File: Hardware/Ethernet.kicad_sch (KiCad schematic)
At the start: 39 parts, among them J1 Conn_01x07_Male, J10 SPI, J2 Conn_01x04_Male, J3 Conn_01x02_Male, J4 Conn_01x02_Male, J5 Conn_01x02_Male, J6 Conn_01x02_Male, J7 Conn_01x08_Male, J8 SPI, J9 QWIIC_Stackable, U1 W5500, Y1 25MHz_SMD_Crystal_Resonator

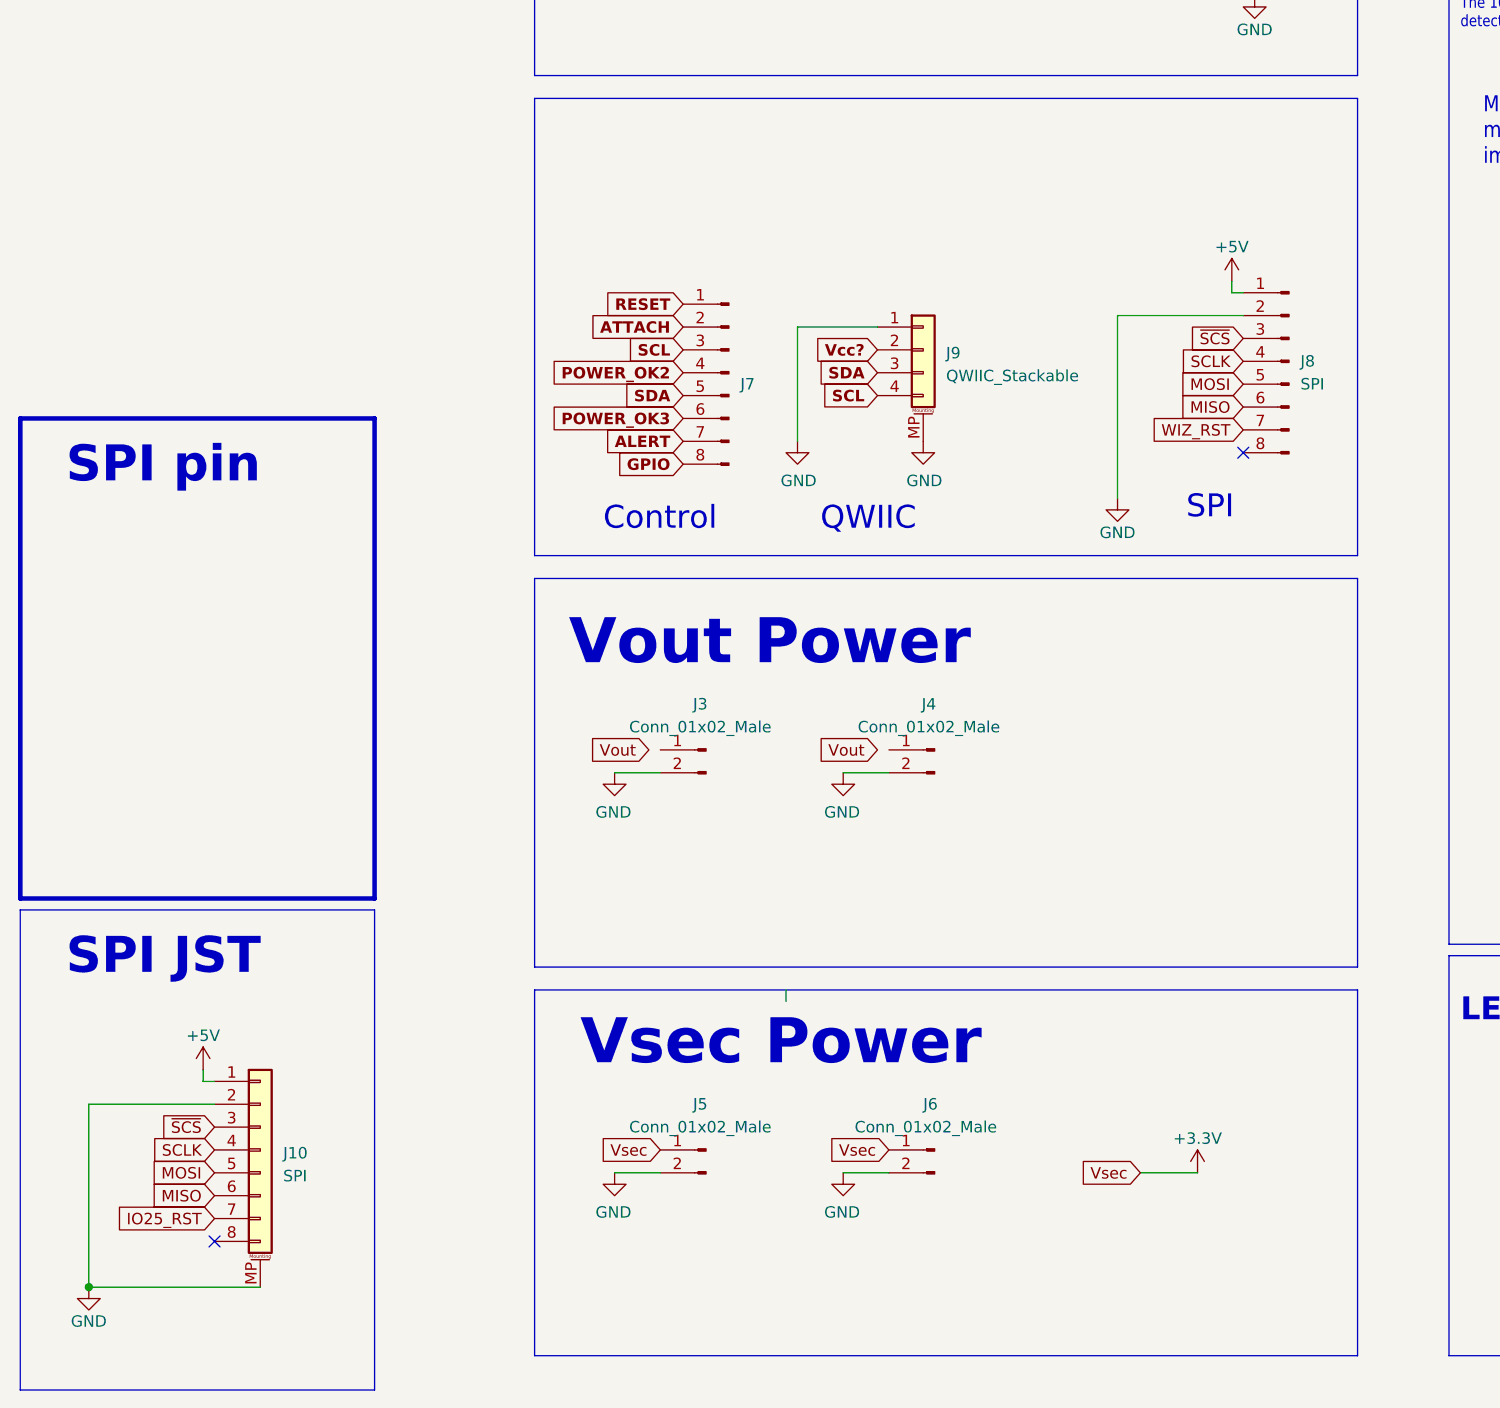
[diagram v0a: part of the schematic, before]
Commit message: Working on SPI
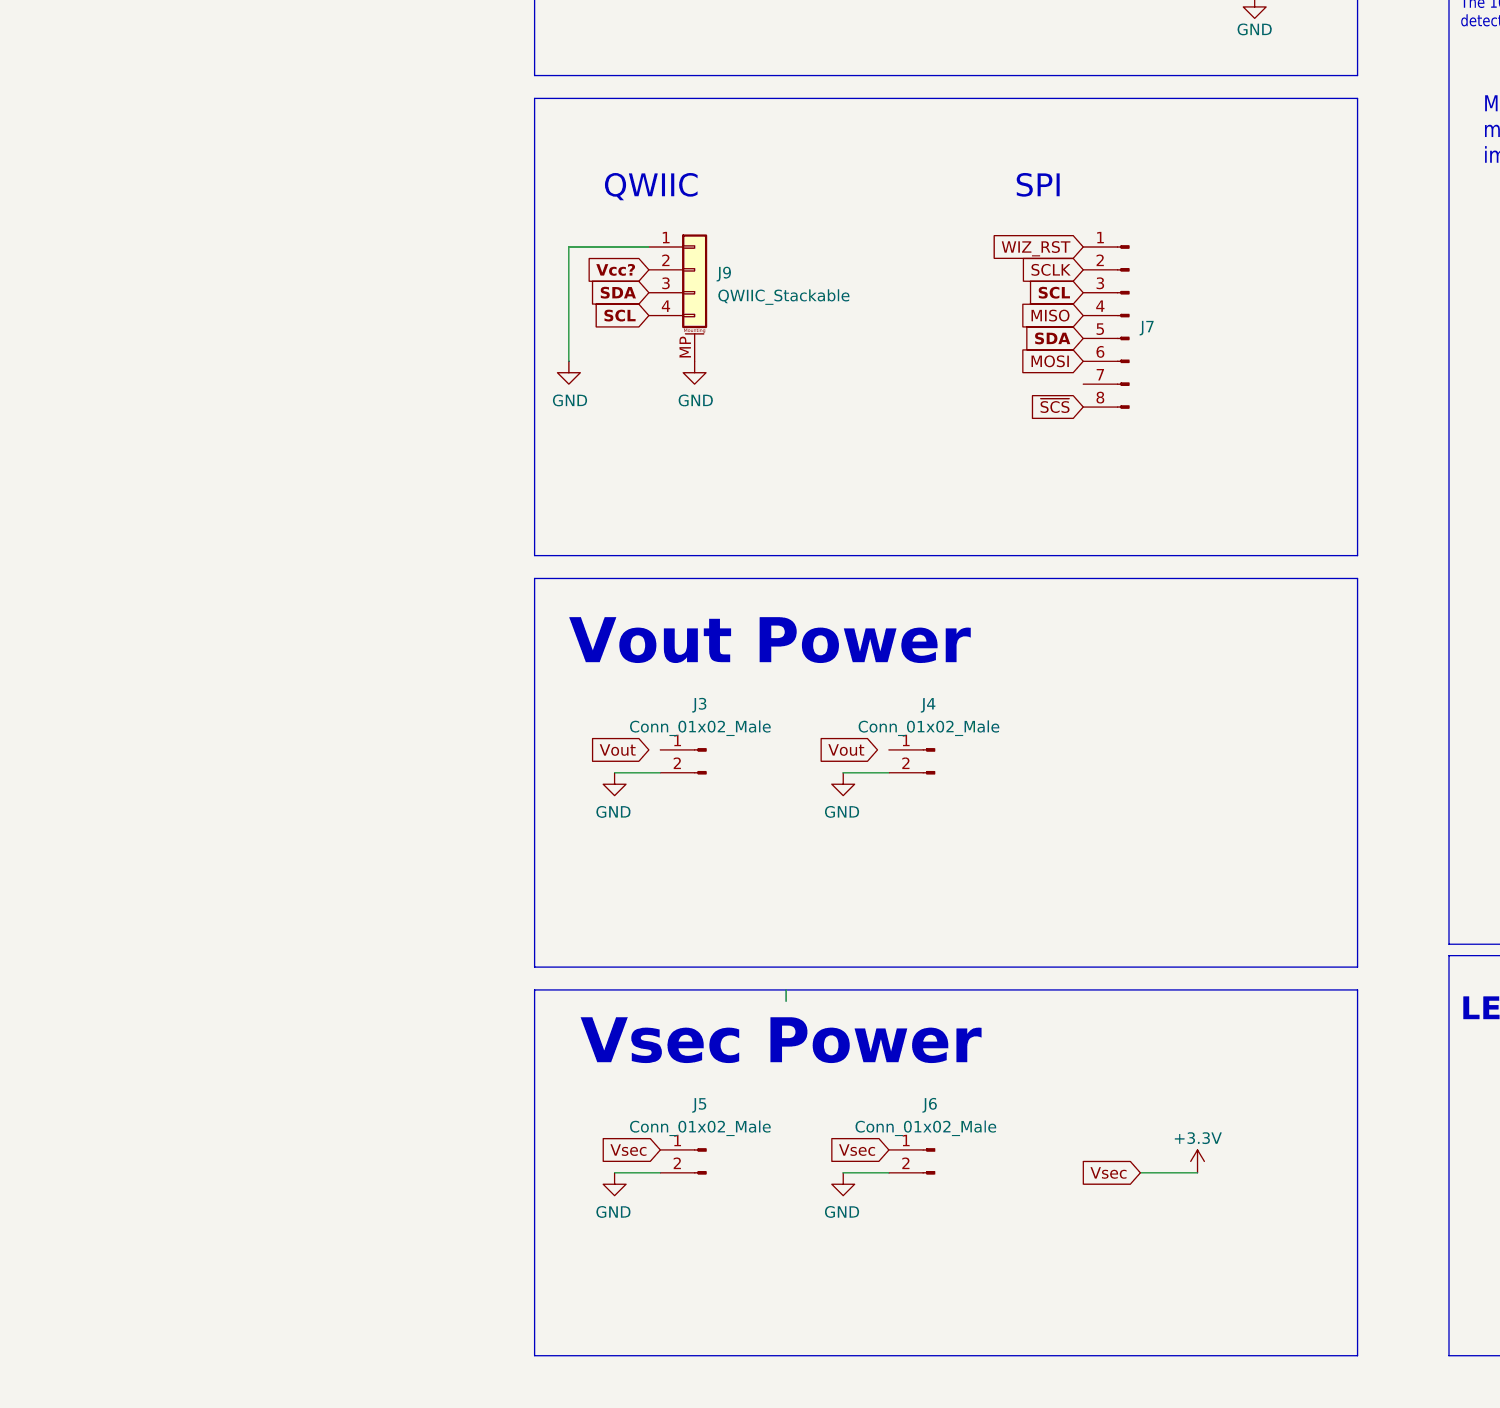
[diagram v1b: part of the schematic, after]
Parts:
- removed J10: SPI, bare-footprints:8 pin jst 1.25 vertical, symbol Connector_Generic_MountingPin:Conn_01x08_MountingPin
- removed J8: SPI, Tinker:PinHeader_1x08_P1.27mm_Vertical, symbol Connector:Conn_01x08_Male
- J7: now in the parts list
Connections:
- net ATTACH is gone; now on net SCLK: J7.2 (Pin_2)
- net GPIO is gone; now on net ~{SCS}: J7.8 (Pin_8)
- net POWER_OK2 is gone; now on net MISO: J7.4 (Pin_4)
- net POWER_OK3 is gone; now on net MOSI: J7.6 (Pin_6)
- net RESET is gone; now on net WIZ_RST: J7.1 (Pin_1)
- net ALERT: no longer names the net of J7.7 (Pin_7)
- no-connect marks 5 -> 3
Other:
- note removed: "Control"
- note removed: "SPI JST"
- note removed: "SPI pin"
- moved on the sheet: J7, J9
